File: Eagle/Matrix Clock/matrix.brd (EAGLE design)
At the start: 173.7 x 50.8 mm, 63 parts, among them IC1 74HC595N, IC2 74HC595N, IC3 74HC595N, IC4 74HC595N, IC5 74HC595N

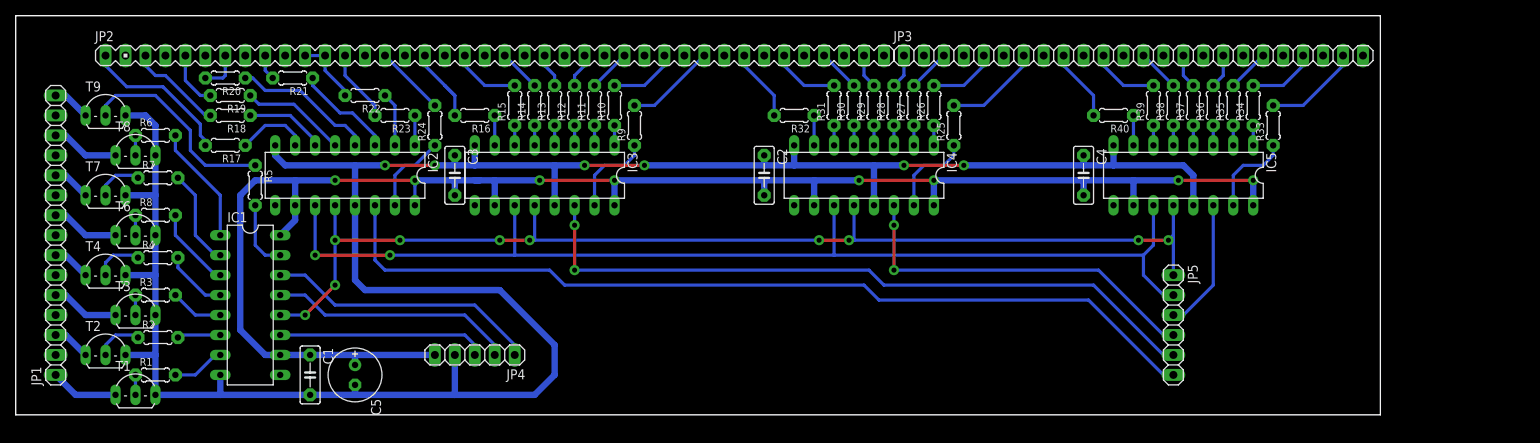
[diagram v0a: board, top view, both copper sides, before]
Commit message: optymalizacja, UART
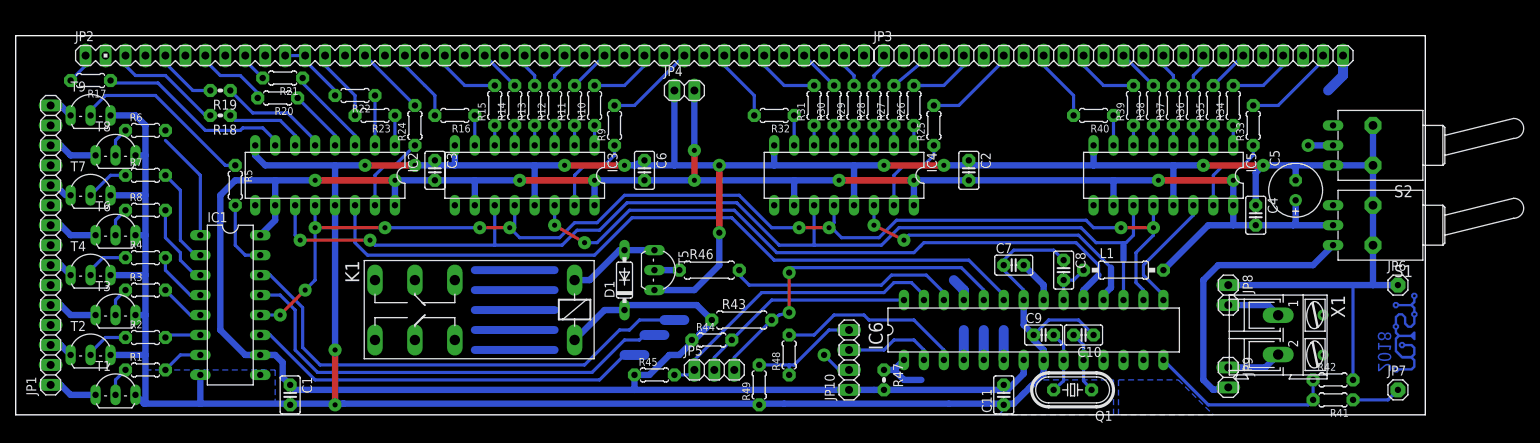
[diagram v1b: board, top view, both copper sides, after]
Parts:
- added C10, C9: (no value), resistor:C025-025X050
- added C11, C6, C7, C8: 100n, resistor:C025-025X050
- added D1: 1N4148DO35-7, diode:DO35-7
- added IC6: MEGA8-P, atmel:DIL28-3
- added JP10: (no value), pinhead:1X04
- added JP6, JP7: (no value), pinhead:1X01
- added JP8, JP9: (no value), pinhead:1X02
- added K1: 4052, relay:F4052
- added L1: (no value), resistor:0207/10
- added Q1: 20MHz, crystal:HC49/S
- added R41, R42, R49: 5k, resistor:0204/5
- added R43: 10k, resistor:0207/7
- added R44: 10k, resistor:0204/5
- added R45: (no value), resistor:0204/5
- added R46: 2k, resistor:0207/7
- added R47: 5k, resistor:0204V
- added R48: 2k, resistor:0204/5
- added S1, S2: (no value), switch:9070-1W
- added T5: (no value), transistor:TO92-CBE
- added U$1: (no value), logo:MIST
- added X1: (no value), con-ptr500:AK300/2
- C1, C2, C3, C4: value (none) -> 100n; device resistor:C050-025X075 -> resistor:C025-025X050
- JP4: device pinhead:1X05 -> pinhead:1X02
- JP5: device pinhead:1X06 -> pinhead:1X03
- R1, R2, R3, R4, R5, R6, R7, R8: value (none) -> 500
- R10, R11, R12, R13, R14, R15, R16, R17, R20, R22, R23, R24, R25, R26, R27, R28, R29, R31, R32, R33, R34, R35, R37, R38, R39, R40, R9: value (none) -> 220
- R18, R19: value (none) -> 220; device resistor:0204/5 -> resistor:0204V
- moved C5 122.0 mm to (162.9, 28.6), turned to 90 degrees
- moved JP5 58.7 mm to (88.9, 5.71), turned to 0 degrees
- moved JP4 42.9 mm to (85.1, 41.3), turned to 0 degrees
- moved C2 26.0 mm to (121.3, 31.1)
- moved C4 22.5 mm to (157.8, 25.4)
- moved R17 19.0 mm to (9.53, 42.5)
- moved R20 7.13 mm to (33.3, 40.3)
- moved C1 3.59 mm to (34.9, 2.54)
- moved C3 2.62 mm to (53.3, 31.1)
- moved JP3 2.54 mm to (139.7, 45.7)
- moved R33 2.54 mm to (157.5, 36.8)
- moved R37 2.54 mm to (147.3, 39.4)
- moved IC3 2.54 mm to (64.8, 30.5)
- moved IC4 2.54 mm to (105.4, 30.5)
- moved R10 2.54 mm to (73.7, 39.4)
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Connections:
- removed net IN_CLK: IC2.11, IC3.11, IC4.11, IC5.11, JP5.2
- removed net SX_CLK: IC1.11, JP4.3
- removed net X_INPUT: IC1.14, JP4.1
- removed net X_RESET: IC1.13, JP4.2
- removed net Y0_IN: IC2.14, JP5.6
- removed net Y1_IN: IC3.14, JP5.5
- removed net Y2_IN: IC4.14, JP5.4
- removed net Y3_IN: IC5.14, JP5.3
- removed net Y_CLK: IC1.12, IC2.12, IC3.12, IC4.12, IC5.12, JP5.1
- new net FOTO: IC6.25, JP3.24
- new net GND_B: JP10.2, S2.2
- new net INPUT: IC6.14, R41.2, R42.1
- new net LATCH: IC1.12, IC2.12, IC3.12, IC4.12, IC5.12, IC6.16
- new net N$11: JP8.2, X1.1
- new net N$14: JP7.1, R41.1
- new net N$2: JP9.1, X1.2
- new net N$36: JP9.2, S1.3
- new net N$41: C9.2, IC6.9, Q1.2
- new net N$42: C10.2, IC6.10, Q1.1
- new net N$43: C7.2, IC6.21
- new net N$52: C8.2, IC6.20, L1.1
- new net N$53: D1.A, K1.2, T5.C
- new net N$54: R46.1, T5.B
- new net N$56: IC6.1, R47.1
- new net N$57: IC6.3, R48.2
- new net RELAY: IC6.26, R46.2
- new net RX: IC6.2, JP10.3
- new net SCL: IC6.28, JP5.2, R44.2
- new net SDA: IC6.27, JP5.1, R45.2
- new net SQW: IC6.24, JP5.3, R43.2
- new net TX: JP10.4, R48.1, R49.2
- new net X0_DATA: IC2.14, IC6.23
- new net X1_DATA: IC3.14, IC6.19
- new net X2_DATA: IC4.14, IC6.18
- new net X3_DATA: IC5.14, IC6.15
- new net X_CLK_DATA: IC2.11, IC3.11, IC4.11, IC5.11, IC6.17
- new net Y_CLK_DATA: IC1.11, IC6.4
- new net Y_DATA: IC1.14, IC6.6
- new net Y_RESET: IC1.13, IC6.5
- net GND: now also C10.1, C11.1, C6.1, C7.1, C8.1, C9.1, IC6.22, IC6.8, JP4.1, JP6.1, JP8.1, R42.2, R49.1, S1.B, S1.B1, S2.3, S2.B, S2.B1, T5.E; no longer JP4.4
- net VCC: now also C11.2, C6.2, D1.C, IC6.7, JP10.1, JP4.2, K1.1, L1.2, R43.1, R44.1, R45.1, R47.2, S1.2; no longer JP4.5
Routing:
- net GND: track 309.6 -> 520.6 mm, vias 6 -> 12
- net VCC: track 215.0 -> 372.3 mm, vias 8 -> 9
- net LATCH: track 0.00 -> 153.6 mm, vias 0 -> 10
- net Y_CLK: track 144.7 -> 0.00 mm, vias 10 -> 0
- net X_CLK_DATA: track 0.00 -> 139.5 mm, vias 0 -> 2
- net IN_CLK: track 138.7 -> 0.00 mm, vias 2 -> 0
- net Y0_IN: track 115.9 -> 0.00 mm
- net X0_DATA: track 0.00 -> 95.9 mm
- net Y1_IN: track 88.9 -> 0.00 mm, vias 2 -> 0
- net X1_DATA: track 0.00 -> 83.2 mm, vias 0 -> 2
- net Y_DATA: track 0.00 -> 69.1 mm
- net Y_RESET: track 0.00 -> 64.9 mm
- net Y_CLK_DATA: track 0.00 -> 56.4 mm
- net Y2_IN: track 47.2 -> 0.00 mm, vias 2 -> 0
- net SQW: track 0.00 -> 45.4 mm, vias 0 -> 2
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- added copper zone on layer 16, net GND
- added copper zone on layer 16, net N$38
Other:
- board size 173.7 x 50.8 mm -> 179.4 x 48.2 mm
- board text added: "2018"
